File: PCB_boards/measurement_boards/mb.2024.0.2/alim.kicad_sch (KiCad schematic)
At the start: 3 parts

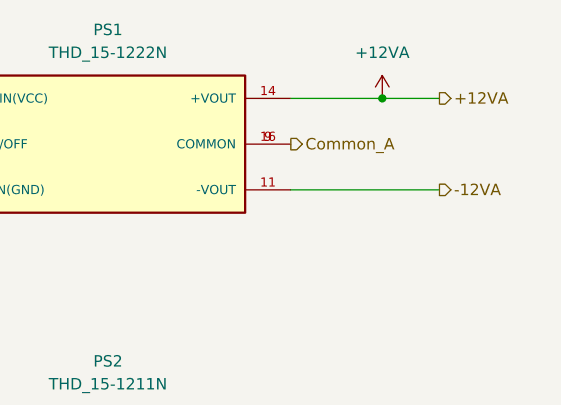
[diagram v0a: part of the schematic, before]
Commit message: update measurement board
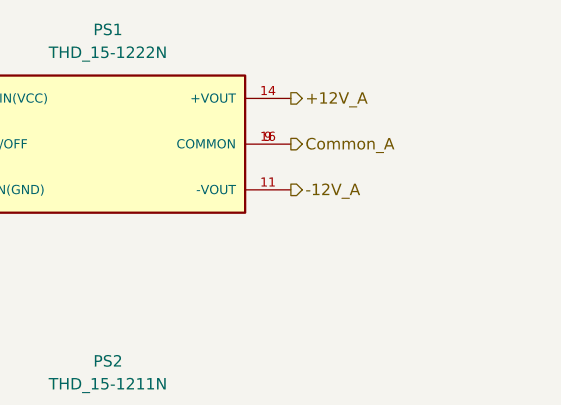
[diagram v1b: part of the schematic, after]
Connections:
- net +12VA renamed +12V_A
- net -12VA renamed -12V_A
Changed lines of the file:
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@@
     (title "Alimentations ")
-  )
-  (junction (at 137.16 40.64) (diameter 0) (color 0 0 0 0)
   )
   (no_connect (at 81.28 87.63))
@@
     (stroke (width 0) (type default))
   )
-  (wire (pts (xy 137.16 40.64) (xy 143.51 40.64))
-    (stroke (width 0) (type default))
-  )
   (wire (pts (xy 81.28 119.38) (xy 81.28 121.92))
     (stroke (width 0) (type default))
   )
-  (wire (pts (xy 127 50.8) (xy 143.51 50.8))
-    (stroke (width 0) (type default))
-  )
   (wire (pts (xy 132.08 116.84) (xy 132.08 119.38))
-    (stroke (width 0) (type default))
-  )
-  (wire (pts (xy 127 40.64) (xy 137.16 40.64))
     (stroke (width 0) (type default))
   )
@@
     (effects (font (size 1.27 1.27)) (justify left))
   )
-  (hierarchical_label "-12VA" (shape output) (at 143.51 50.8 0) (fields_autoplaced)
+  (hierarchical_label "-12V_A" (shape output) (at 127 50.8 0) (fields_autoplaced)
     (effects (font (size 1.27 1.27)) (justify left))
   )
@@
     (effects (font (size 1.27 1.27)) (justify left))
   )
-  (hierarchical_label "+12VA" (shape output) (at 143.51 40.64 0) (fields_autoplaced)
+  (hierarchical_label "+12V_A" (shape output) (at 127 40.64 0) (fields_autoplaced)
     (effects (font (size 1.27 1.27)) (justify left))
   )
@@
         )
       )
-    )
-  )
-  (symbol (lib_id "power:+12VA") (at 137.16 40.64 0) (unit 1)
-    (in_bom yes) (on_board yes) (dnp no) (fields_autoplaced)
-    (property "Reference" "#PWR04" (at 137.16 44.45 0)
-      (effects (font (size 1.27 1.27)) hide)
-    )
-    (property "Value" "+12VA" (at 137.16 35.56 0)
-      (effects (font (size 1.27 1.27)))
-    )
-    (property "Footprint" "" (at 137.16 40.64 0)
-      (effects (font (size 1.27 1.27)) hide)
-    )
-    (property "Datasheet" "" (at 137.16 40.64 0)
-      (effects (font (size 1.27 1.27)) hide)
-    )
-    (pin "1")
-    (instances
-      (project "mb.2024.0.2"
-        (path "/62d2b953-c7cc-4d07-805d-38225011d95a/9f60bb1d-ca92-41d5-b592-f34396aa7479"
-          (reference "#PWR04") (unit 1)
-        )
-      )
